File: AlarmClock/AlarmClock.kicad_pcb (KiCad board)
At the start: 2 copper layers, 39 parts, among them Q1 2N3904, Q2 2N3904, Q3 2N3904, Q4 2N3904, Q5 2N3904, SW1 SW_Push_Dual, SW2 SW_Push_Dual, SW3 SW_Push_Dual, SW4 SW_Push_Dual, SW5 SW_Push_Dual, U1 LM386, U2 LTC-4727JR, U3 LM358

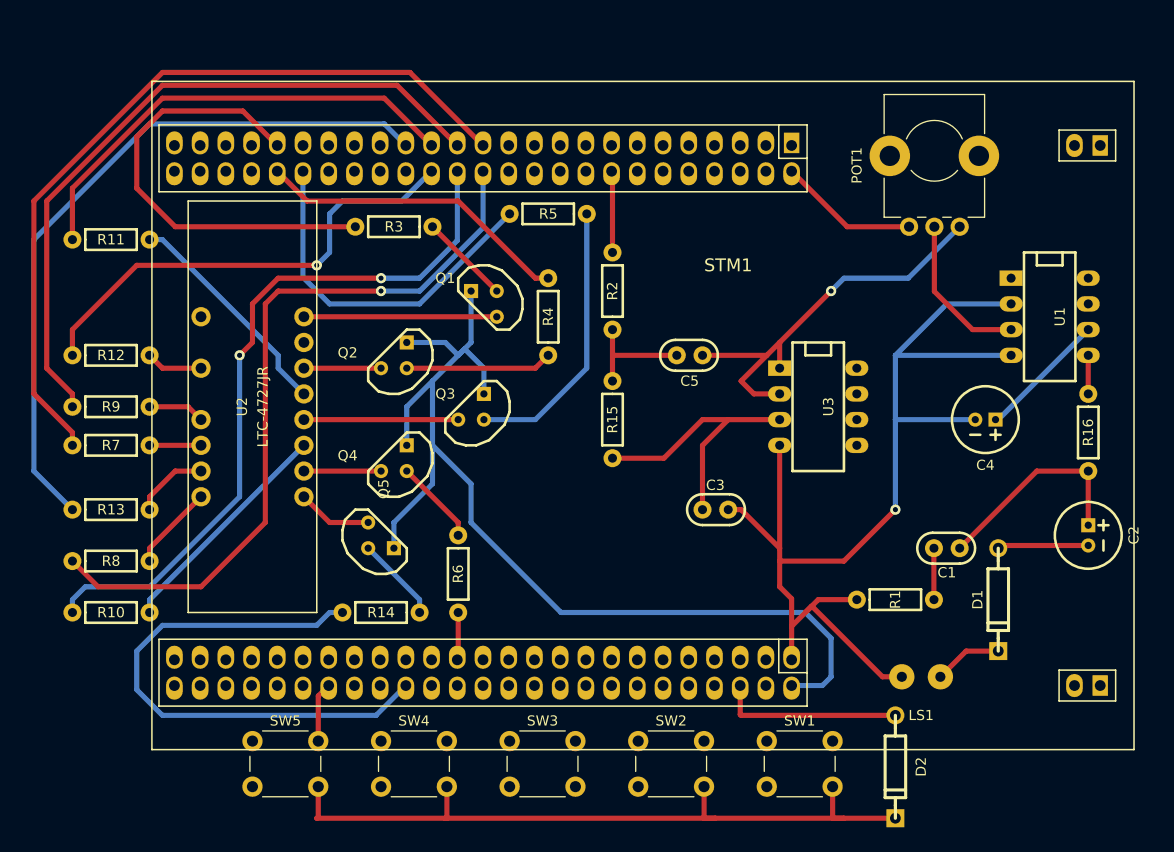
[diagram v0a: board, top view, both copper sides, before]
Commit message: geber files and final pcb
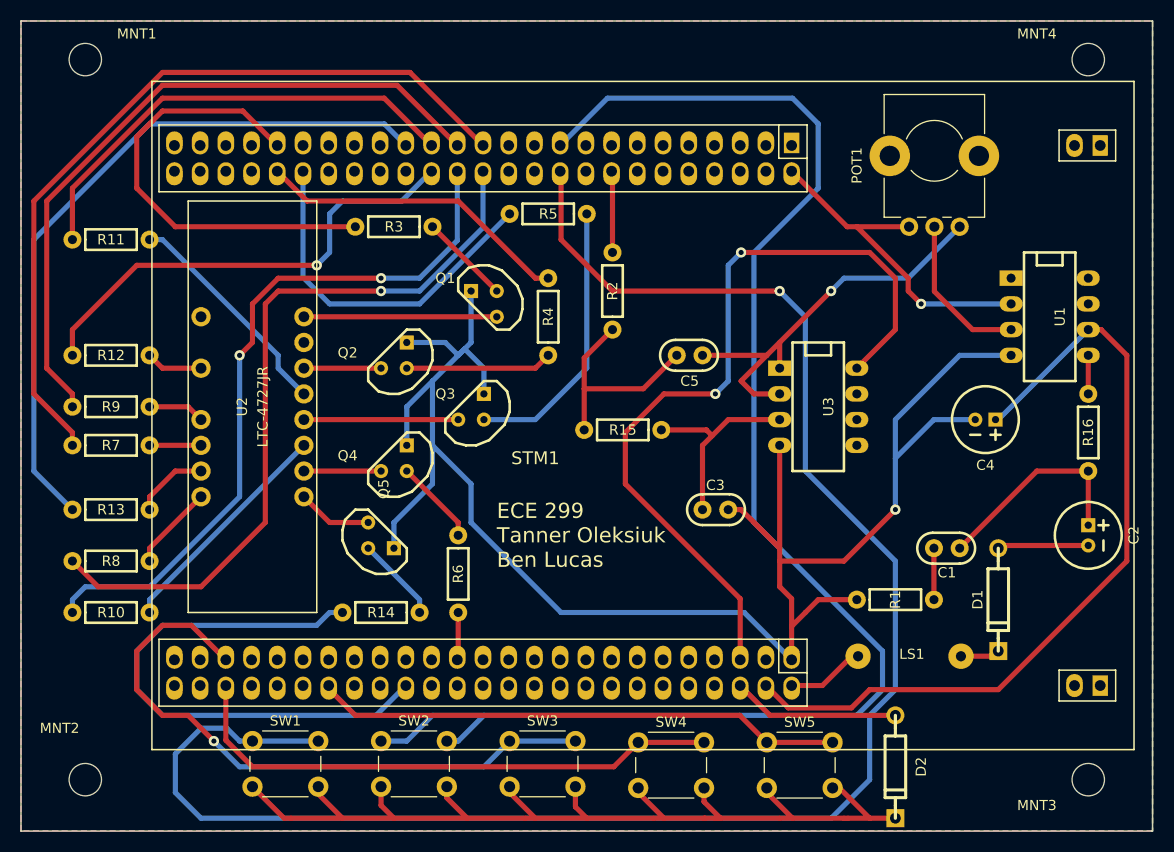
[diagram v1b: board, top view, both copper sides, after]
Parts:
- added MNT1: MountingHole_3.2mm_M3, Mounting_Holes:MountingHole_3.2mm_M3, F.Cu at (94.0, 71.1)
- added MNT2: MountingHole_3.2mm_M3, Mounting_Holes:MountingHole_3.2mm_M3, F.Cu at (94.0, 142.2)
- added MNT3: MountingHole_3.2mm_M3, Mounting_Holes:MountingHole_3.2mm_M3, F.Cu at (193.0, 142.2)
- added MNT4: MountingHole_3.2mm_M3, Mounting_Holes:MountingHole_3.2mm_M3, F.Cu at (193.0, 71.1)
- LS1: footprint Wire_Pads:SolderWirePad_2x_1mmDrill -> Wire_Connections_Bridges:WireConnection_1.00mmDrill
- SW1, SW2, SW3, SW4, SW5: value SW_Push_Dual -> SW_Push
- moved SW5 50.8 mm to (161.3, 138.6)
- moved SW1 50.8 mm to (110.5, 138.4)
- moved SW4 25.4 mm to (148.6, 138.6)
- moved SW2 25.4 mm to (123.2, 138.4)
- moved LS1 4.43 mm to (180.5, 130.0)
- moved R15 1.44 mm to (147.1, 107.7), turned to 180 degrees
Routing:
- net PC4: track 0.00 -> 175.4 mm, vias 0 -> 1
- net PC5: track 0.00 -> 148.6 mm
- net +3V3: track 18.2 -> 96.0 mm, vias 0 -> 2
- net +5V: track 12.8 -> 80.6 mm
- net PC8: track 0.00 -> 62.6 mm, vias 0 -> 1
- net PC9: track 0.00 -> 54.7 mm
- net PC11: track 5.91 -> 52.3 mm
- net Net-(D2-PadK): track 72.1 -> 102.0 mm
- net GND: track 227.4 -> 216.8 mm, vias 1 -> 2
- net Net-(C5-Pad2): track 14.0 -> 21.6 mm
- net Net-(C3-Pad1): track 25.5 -> 20.3 mm
- net Net-(D1-PadK): track 8.67 -> 3.89 mm
- net PA4: track 8.57 -> 8.06 mm
- added copper zone on B.Cu, net GND
- added copper zone on F.Cu, net GND
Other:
- board outline added: 111.8 x 80 mm
- board text added: "ECE 299 Tanner Oleksiuk Ben Lucas"
